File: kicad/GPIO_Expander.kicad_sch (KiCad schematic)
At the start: 12 parts, among them J21 Conn_01x07_Pin, U22 MCP23017_SO

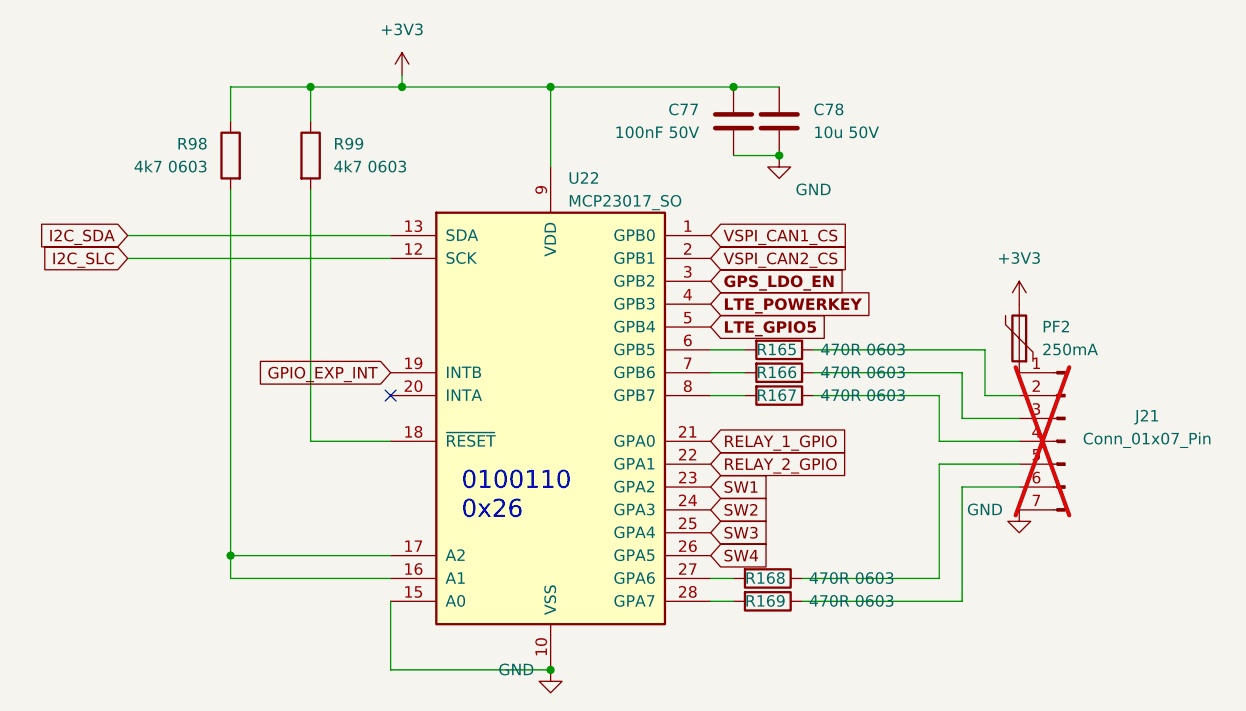
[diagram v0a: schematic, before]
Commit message: WIP
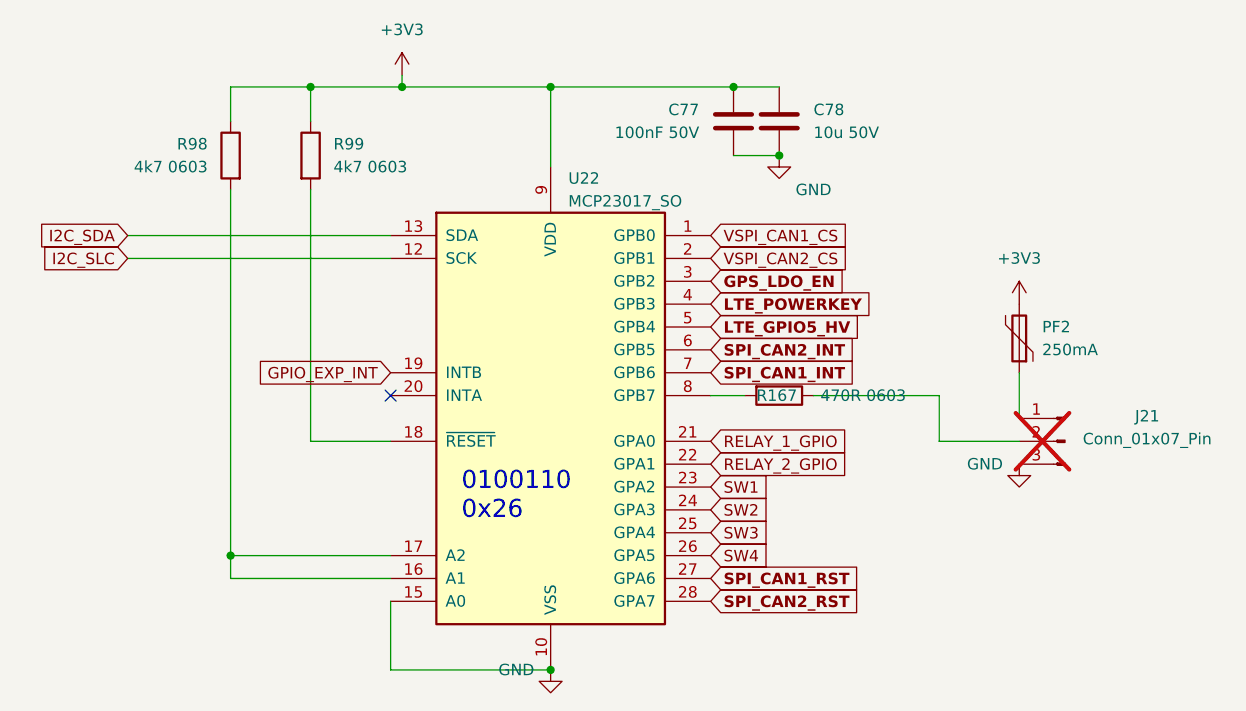
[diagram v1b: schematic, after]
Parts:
- removed R165, R166, R168, R169: 470R 0603, Resistor_SMD:R_0603_1608Metric, symbol Device:R
- J21: footprint Connector_PinHeader_1.27mm:PinHeader_1x07_P1.27mm_Vertical -> Connector_PinHeader_1.27mm:PinHeader_1x03_P1.27mm_Vertical; symbol Connector:Conn_01x07_Pin -> Connector:Conn_01x03_Pin; now in the parts list
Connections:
- net GND: now also J21.3 (Pin_3); no longer J21.7 (Pin_7)
- net at R167.1: now also J21.2 (Pin_2); no longer J21.4 (Pin_4)
- net SPI_CAN1_RST: now reaches U22.27 (GPA6)
- net SPI_CAN1_INT: now reaches U22.7 (GPB6)
- net SPI_CAN2_INT: now reaches U22.6 (GPB5)
- net SPI_CAN2_RST: now reaches U22.28 (GPA7)
- net LTE_GPIO5 renamed LTE_GPIO5_HV

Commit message: bom cleanup
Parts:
- J21: now left out of the parts list
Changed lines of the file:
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@@
 		(unit 1)
 		(exclude_from_sim no)
-		(in_bom yes)
+		(in_bom no)
 		(on_board yes)
 		(dnp yes)
